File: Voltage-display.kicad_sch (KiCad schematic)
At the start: 25 parts, among them J1 HV+ SOLDER, J2 HV- SOLDER, J3 Conn_01x02, Q1 DMP2035UQ-7, SW1 SW_SPST, U1 AMC1311BQDWVQ1, U2 R05CT05S-R

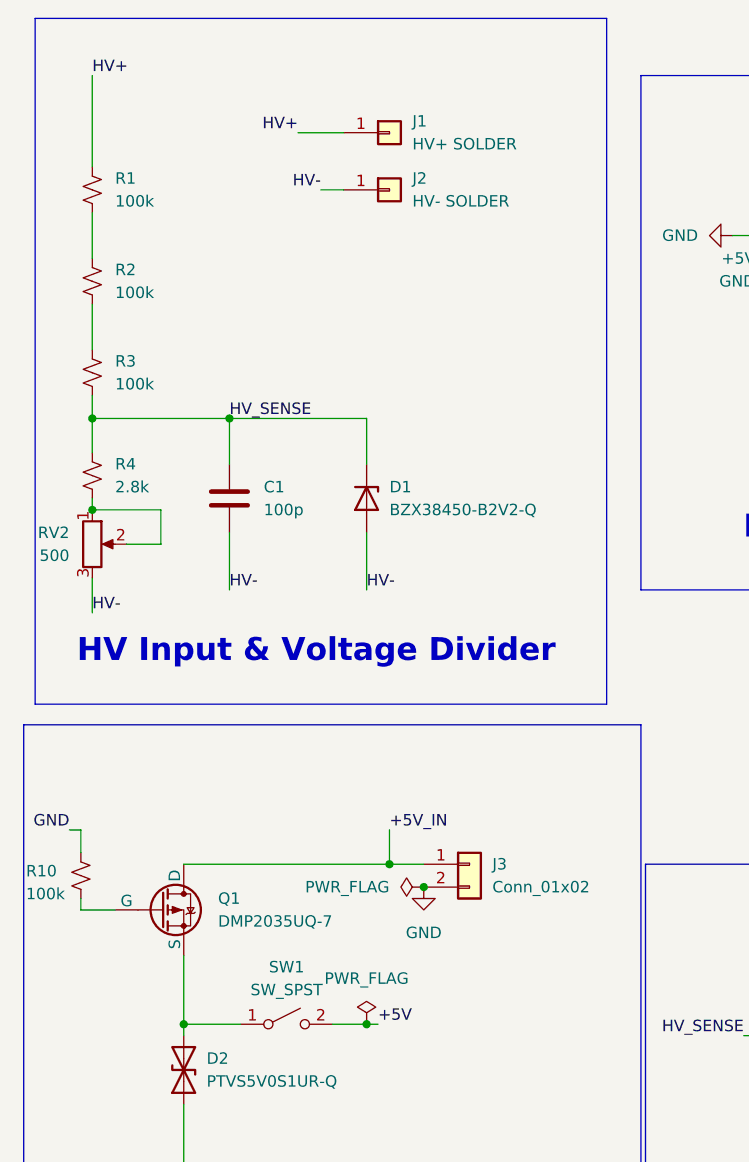
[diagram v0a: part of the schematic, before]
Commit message: Update files
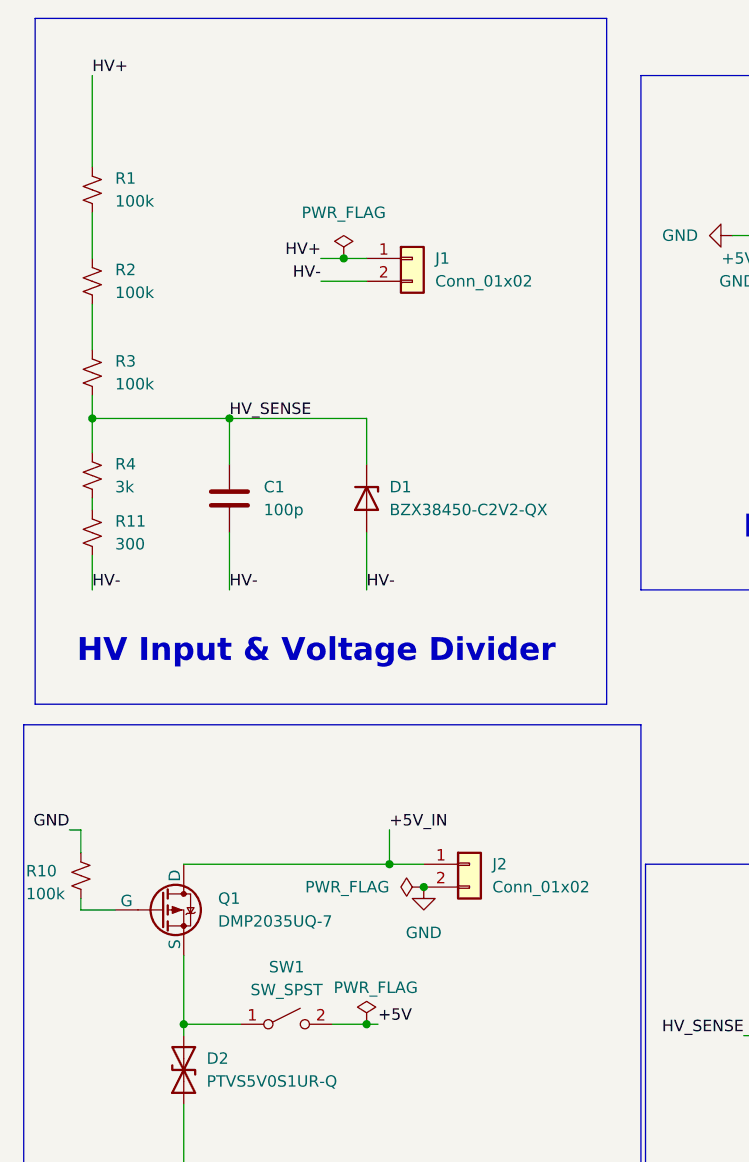
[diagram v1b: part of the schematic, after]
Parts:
- removed J1: HV+ SOLDER, Connector_Wire:SolderWire-0.5sqmm_1x01_D0.9mm_OD2.1mm_Relief, symbol Connector_Generic:Conn_01x01
- removed J2: HV- SOLDER, Connector_Wire:SolderWire-0.5sqmm_1x01_D0.9mm_OD2.1mm_Relief, symbol Connector_Generic:Conn_01x01
- removed RV2: 500, Potentiometer_THT:Potentiometer_Bourns_3296W_Vertical, symbol Device:R_Potentiometer
- added J1: Conn_01x02, Connector_PinHeader_2.54mm:PinHeader_1x02_P2.54mm_Vertical, symbol Connector_Generic:Conn_01x02
- added R11: 300, Resistor_SMD:R_1206_3216Metric_Pad1.30x1.75mm_HandSolder, symbol Device:R_Small_US
- D1: value BZX38450-B2V2-Q -> BZX38450-C2V2-QX
- R4: value 2.8k -> 3k
- renumbered J3 to J2
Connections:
- net HV+: now also J1.1 (Pin_1)
- net HV-: now also J1.2 (Pin_2), R11.2
- net at R4.2: now also R11.1
